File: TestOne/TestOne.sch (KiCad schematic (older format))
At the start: 28 parts, among them SW1 SW_Push, U1 ATmega32U4-AU, Y1 Crystal_GND24_Small

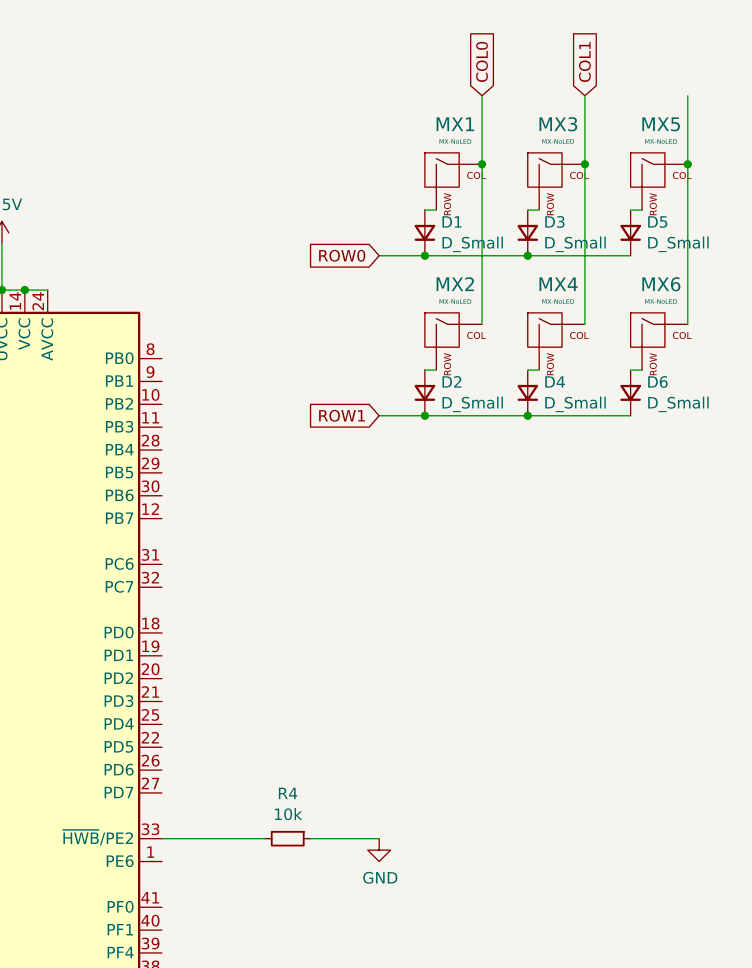
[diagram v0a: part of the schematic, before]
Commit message: Created PCB
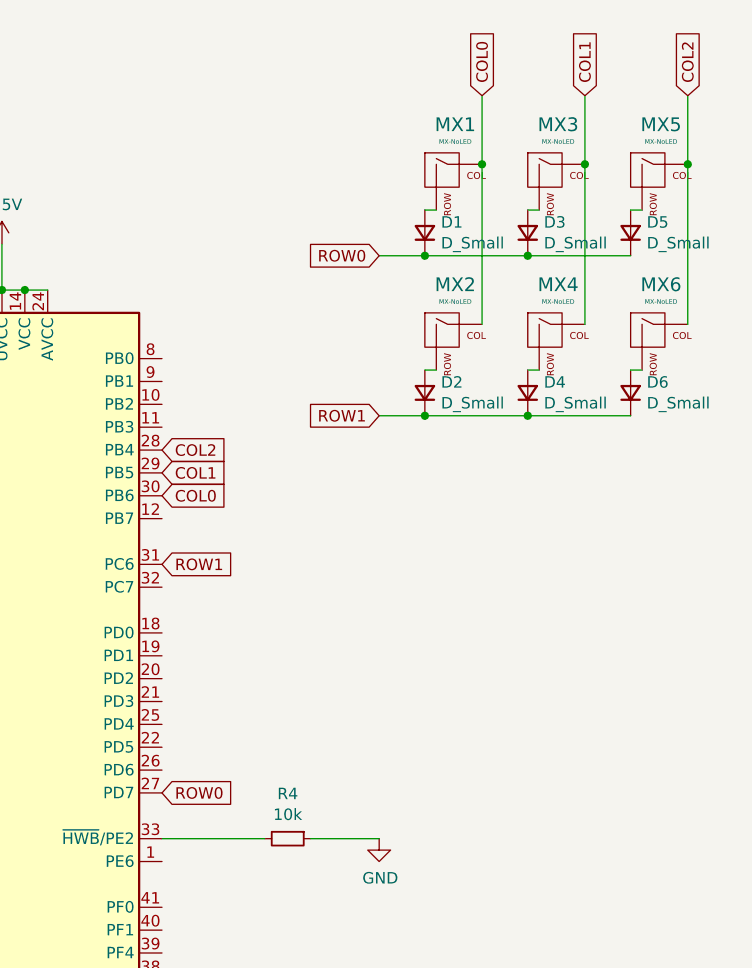
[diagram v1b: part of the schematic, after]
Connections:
- net labels added: COL2
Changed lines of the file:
@@
 Text GLabel 6150 1000 1    50   Input ~ 0
 COL1
+Text GLabel 4300 2650 2    50   Input ~ 0
+COL1
+Text GLabel 4300 2750 2    50   Input ~ 0
+COL0
+Text GLabel 4300 4050 2    50   Input ~ 0
+ROW0
+Text GLabel 4300 3050 2    50   Input ~ 0
+ROW1
+Text GLabel 6600 1000 1    50   Input ~ 0
+COL2
+Text GLabel 4300 2550 2    50   Input ~ 0
+COL2
 $EndSCHEMATC
